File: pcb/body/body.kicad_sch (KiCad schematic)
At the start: 7 parts, among them J1 Conn_01x05_Pin, J2 Conn_01x08_Socket, J3 Output_1_2, J4 Output_3_4, J5 Headphones, J6 AudioJack3_SwitchTR, U1 Teensy4.1

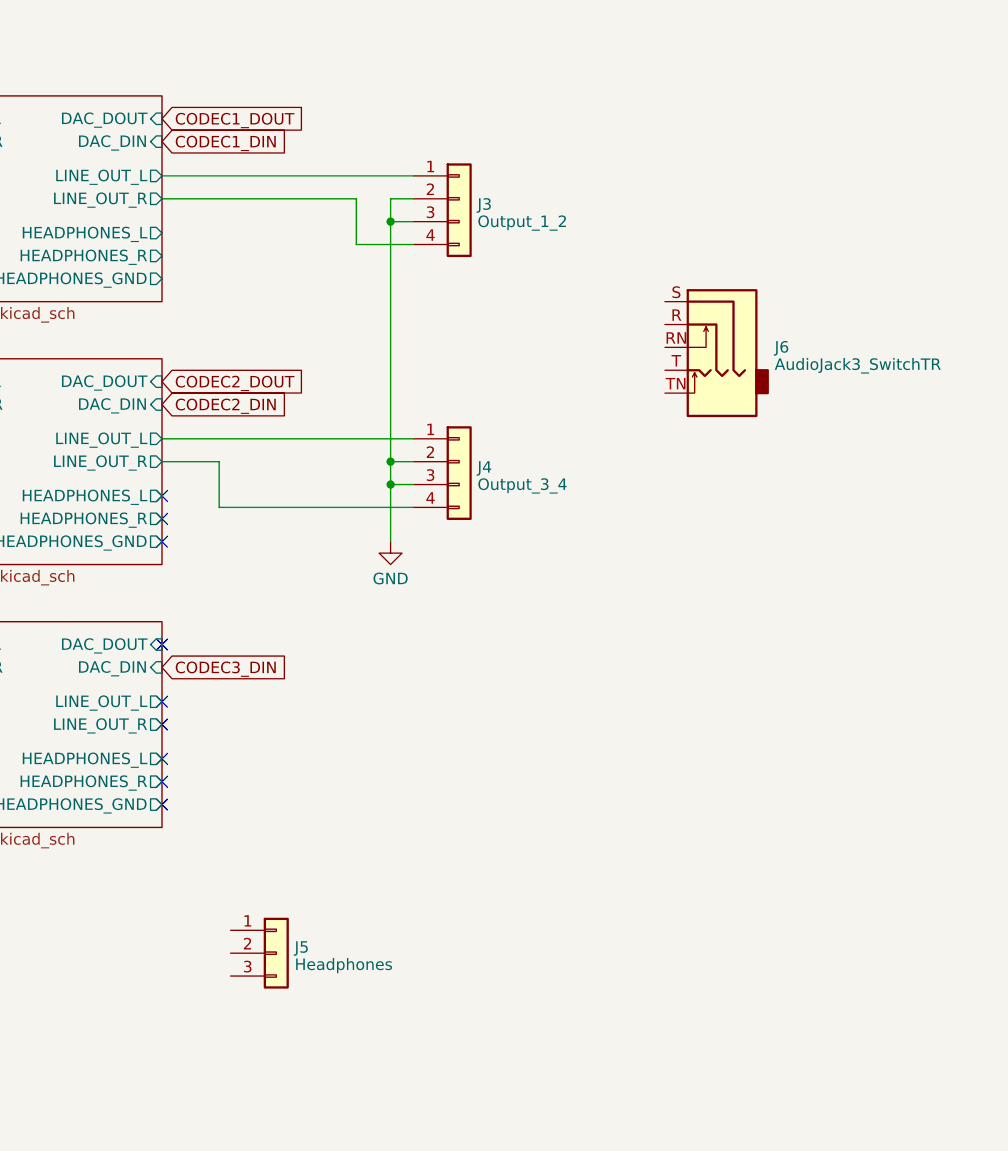
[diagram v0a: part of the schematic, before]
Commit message: initial layout
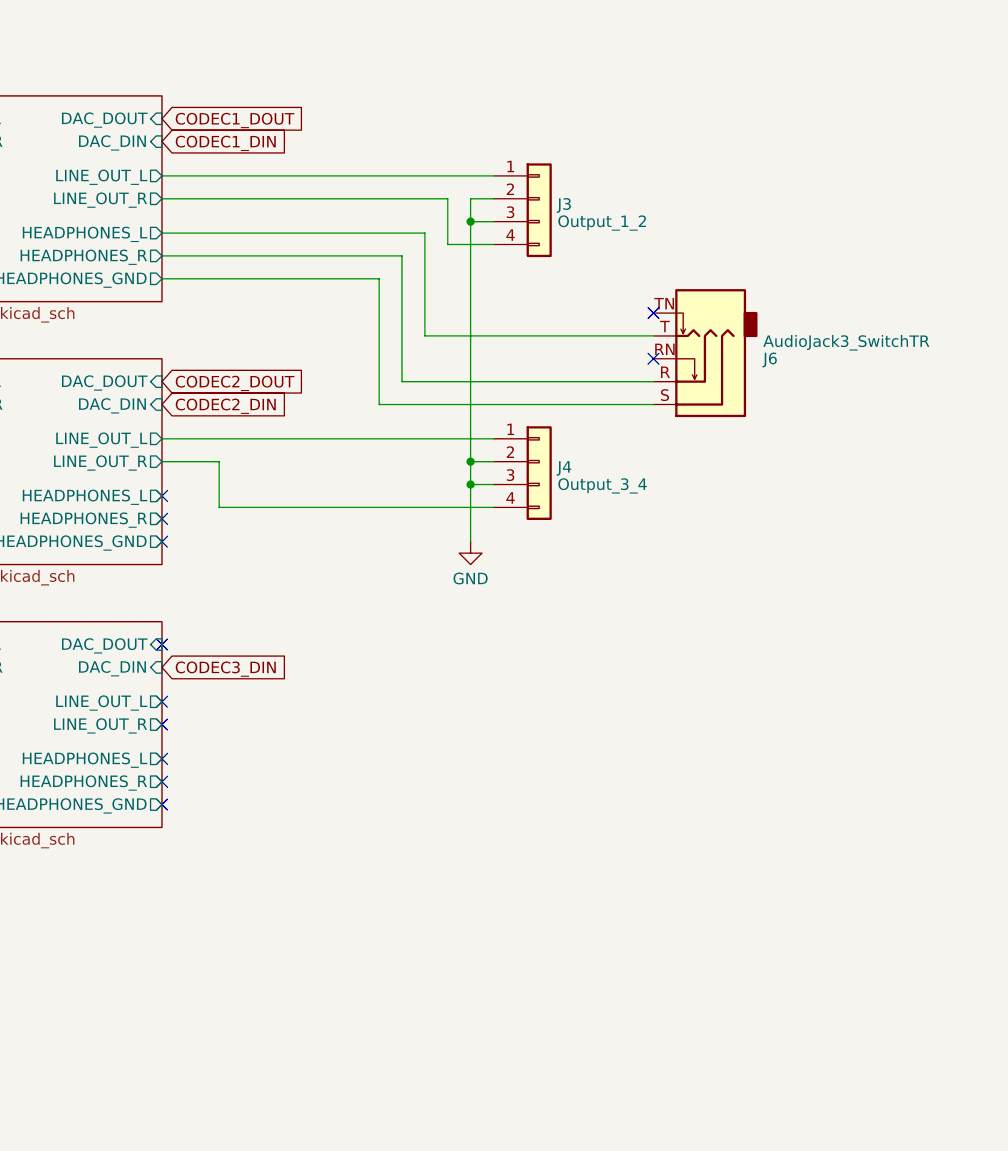
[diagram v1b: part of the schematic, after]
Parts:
- removed J5: Headphones, Connector_PinHeader_2.54mm:PinHeader_1x03_P2.54mm_Vertical, symbol Connector_Generic:Conn_01x03
- J6: footprint (none) -> Connector_Audio:Jack_3.5mm_CUI_SJ1-3525N_Horizontal
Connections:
- net codec1/HEADPHONES_GND: now also J6.S
- net codec1/HEADPHONES_L: now also J6.T
- net codec1/HEADPHONES_R: now also J6.R
- no-connect marks 9 -> 11
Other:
- moved on the sheet: J3, J4, J6

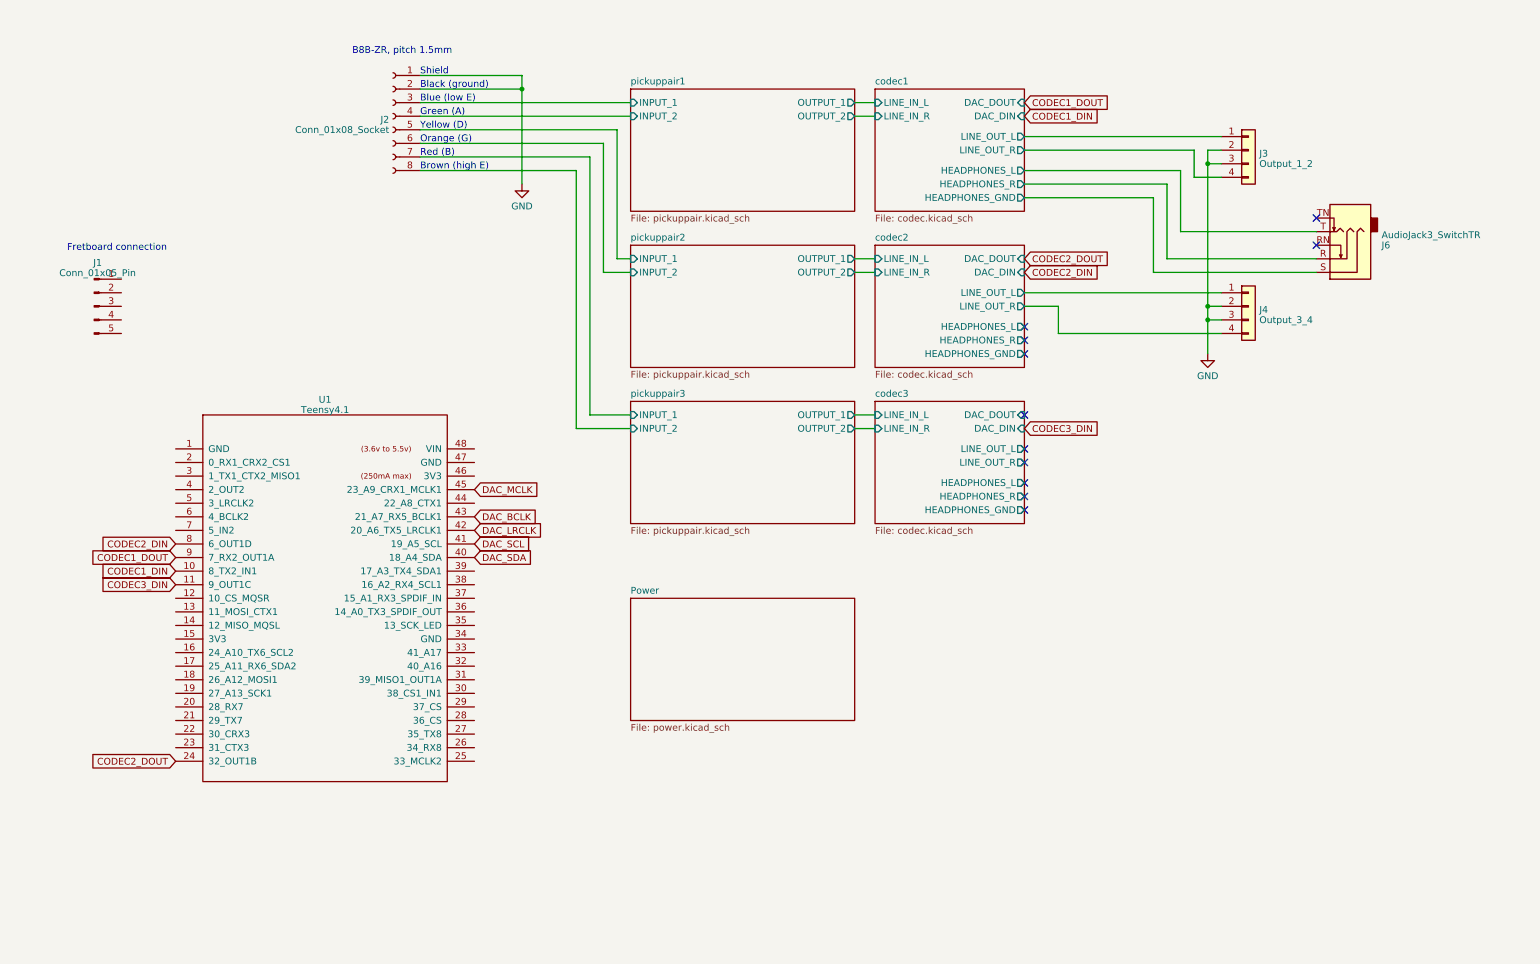
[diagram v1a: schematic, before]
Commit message: lots more layout
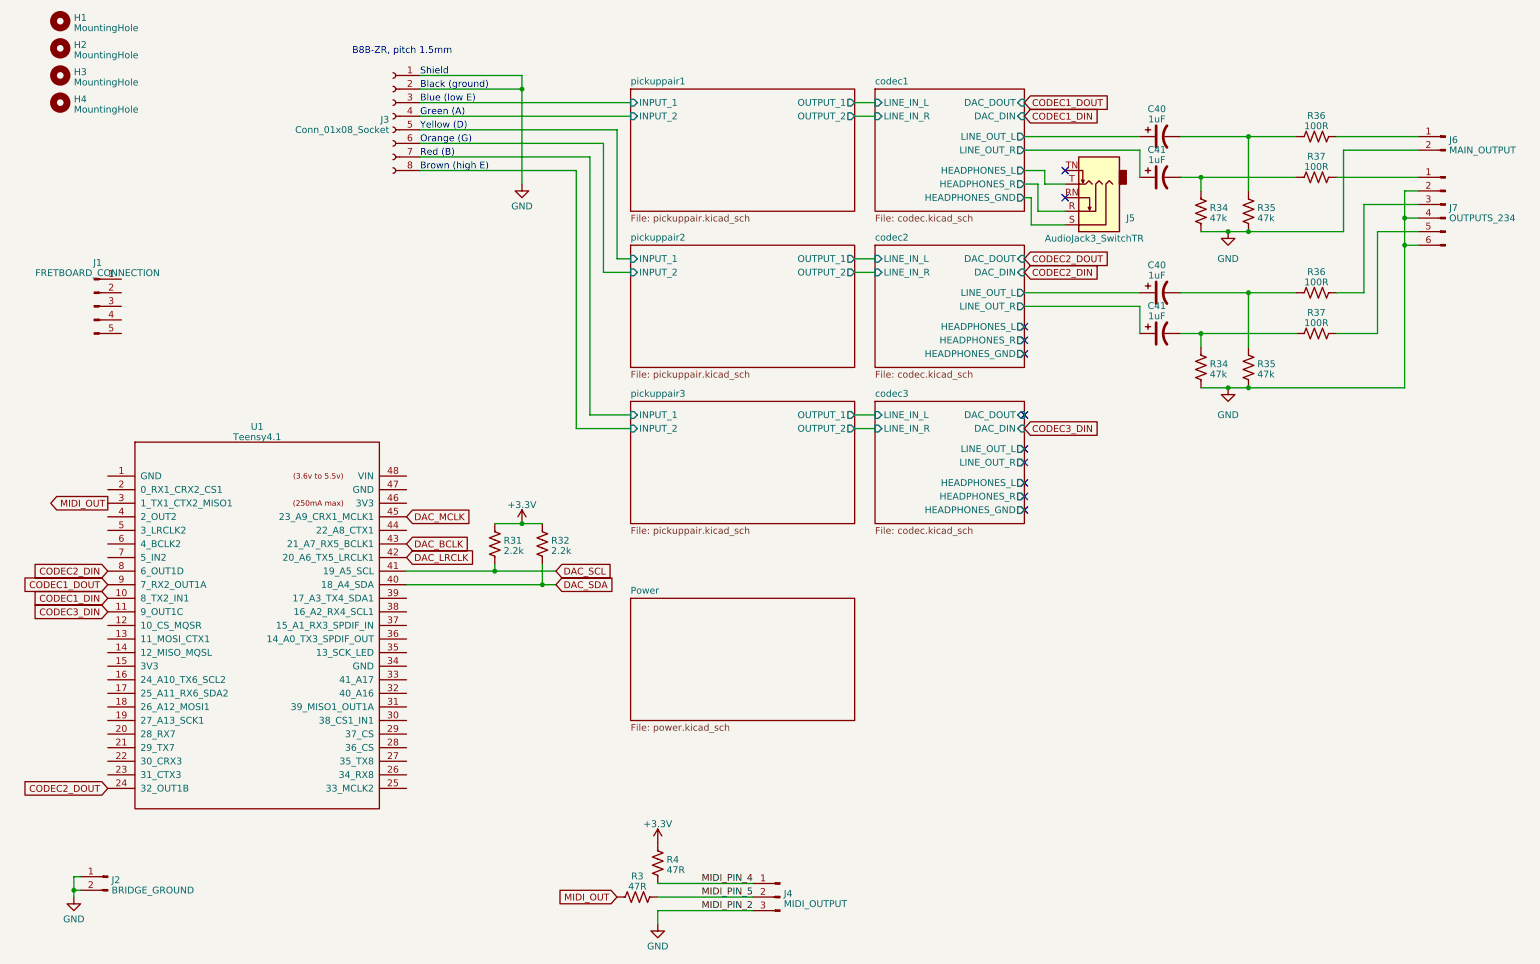
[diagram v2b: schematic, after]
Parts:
- removed J3: Output_1_2, Connector_PinHeader_2.54mm:PinHeader_1x04_P2.54mm_Vertical, symbol Connector_Generic:Conn_01x04
- removed J4: Output_3_4, Connector_PinHeader_2.54mm:PinHeader_1x04_P2.54mm_Vertical, symbol Connector_Generic:Conn_01x04
- removed J6: AudioJack3_SwitchTR, Connector_Audio:Jack_3.5mm_CUI_SJ1-3525N_Horizontal, symbol Connector_Audio:AudioJack3_SwitchTR
- added C40 (x2), C41 (x2): 1uF, Capacitor_SMD:C_0603_1608Metric, symbol Device:C_Polarized_US
- added H1, H2, H3, H4: MountingHole, MountingHole:MountingHole_3.2mm_M3, symbol Mechanical:MountingHole
- added J2: BRIDGE_GROUND, Connector_PinHeader_2.54mm:PinHeader_1x02_P2.54mm_Horizontal, symbol Connector:Conn_01x02_Pin
- added J4: MIDI_OUTPUT, Connector_PinHeader_2.54mm:PinHeader_1x03_P2.54mm_Horizontal, symbol Connector:Conn_01x03_Pin
- added J5: AudioJack3_SwitchTR, Connector_Audio:Jack_3.5mm_CUI_SJ1-3525N_Horizontal, symbol Connector_Audio:AudioJack3_SwitchTR
- added J6: MAIN_OUTPUT, Connector_PinHeader_2.54mm:PinHeader_1x02_P2.54mm_Horizontal, symbol Connector:Conn_01x02_Pin
- added J7: OUTPUTS_234, Connector_PinHeader_2.54mm:PinHeader_1x06_P2.54mm_Vertical, symbol Connector:Conn_01x06_Pin
- added R3, R4: 47R, Resistor_SMD:R_0603_1608Metric, symbol Device:R_US
- added R31, R32: 2.2k, Resistor_SMD:R_0603_1608Metric, symbol Device:R_US
- added R34 (x2), R35 (x2): 47k, Resistor_SMD:R_0603_1608Metric, symbol Device:R_US
- added R36 (x2), R37 (x2): 100R, Resistor_SMD:R_0603_1608Metric, symbol Device:R_US
- J1: value Conn_01x05_Pin -> FRETBOARD_CONNECTION
- renumbered J2 to J3
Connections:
- net DAC_SCL: now also R31.1
- net DAC_SDA: now also R32.1
- net GND: now also J2.1 (Pin_1), J2.2 (Pin_2), J4.3 (Pin_3), J6.2 (Pin_2), J7.2 (Pin_2), J7.4 (Pin_4), J7.6 (Pin_6), R34.1, R34.1, R35.1, R35.1
- net codec1/HEADPHONES_GND: now also J5.S
- net codec1/HEADPHONES_L: now also J5.T
- net codec1/HEADPHONES_R: now also J5.R
- net codec1/LINE_OUT_L: now also C40.1
- net codec1/LINE_OUT_R: now also C41.1
- net codec2/LINE_OUT_L: now also C40.1
- net codec2/LINE_OUT_R: now also C41.1
- net MIDI_OUT: now reaches U1.3 (1_TX1_CTX2_MISO1)
- net MIDI_OUT: now also R3.1
- new net: J7.1 (Pin_1), R37.1
- new net: J7.3 (Pin_3), R36.1
- new net: J7.5 (Pin_5), R37.1
- new net: J6.1 (Pin_1), R36.1
- new net: C41.2, R34.2, R37.2 (x2)
- new net: C40.2, R35.2, R36.2 (x2)
- new net +3.3V: R31.2, R32.2, R4.1
- new net MIDI_PIN_4: J4.1 (Pin_1), R4.2
- new net MIDI_PIN_5: J4.2 (Pin_2), R3.2
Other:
- note removed: "Fretboard connection"
- moved on the sheet: U1
